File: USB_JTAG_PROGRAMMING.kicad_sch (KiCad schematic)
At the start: 85 parts, among them J16 10118194-0001LF, U3 FT2232HQ, U36 MIC5504-3.3YM5-TR, U37 93LC56BT-I/OT, U38 KC2016K12.0000C1GE00, U39 SN74LVC1T45DBVR, U40 NC7WZ07P6X, U41 NC7SZ125M5X, U42 SN74LVC1T45DBVR, U43 SN74LVC1T45DBVR, U44 SN74LVC1T45DBVR, U45 SN74LVC1T45DBVR, U46 NC7WZ126K8X, U47 NC7WZ126K8X

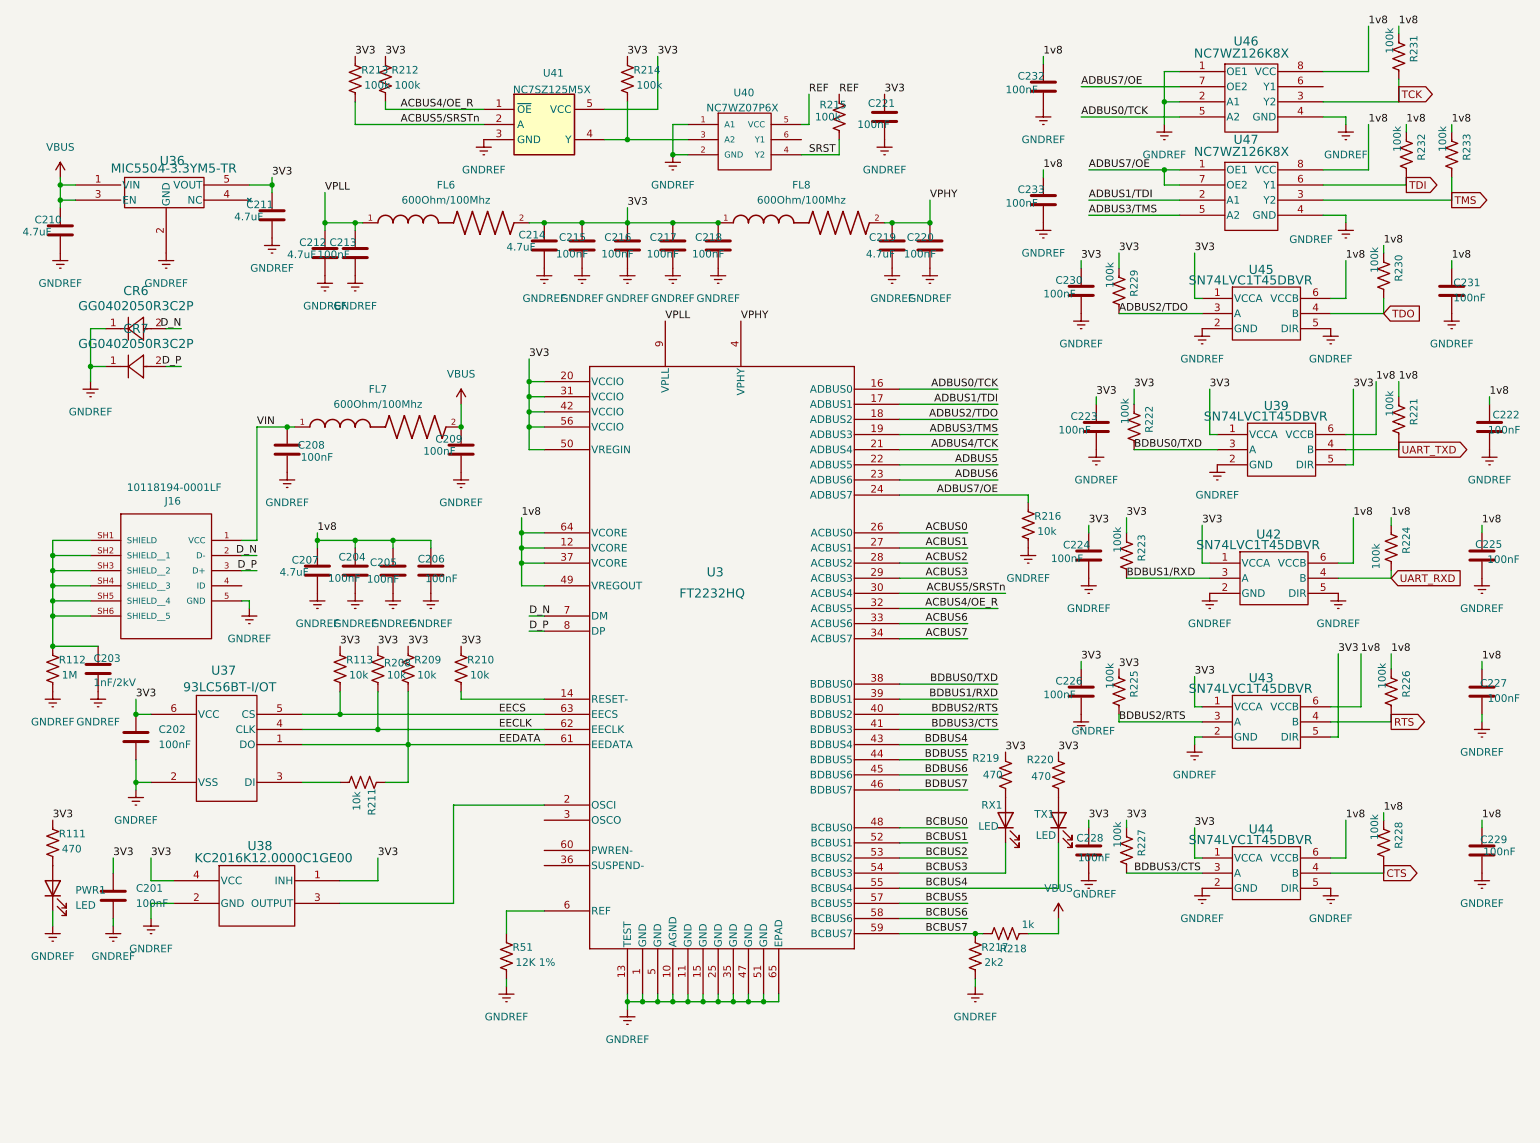
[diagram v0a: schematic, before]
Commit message: ready for manufacturing
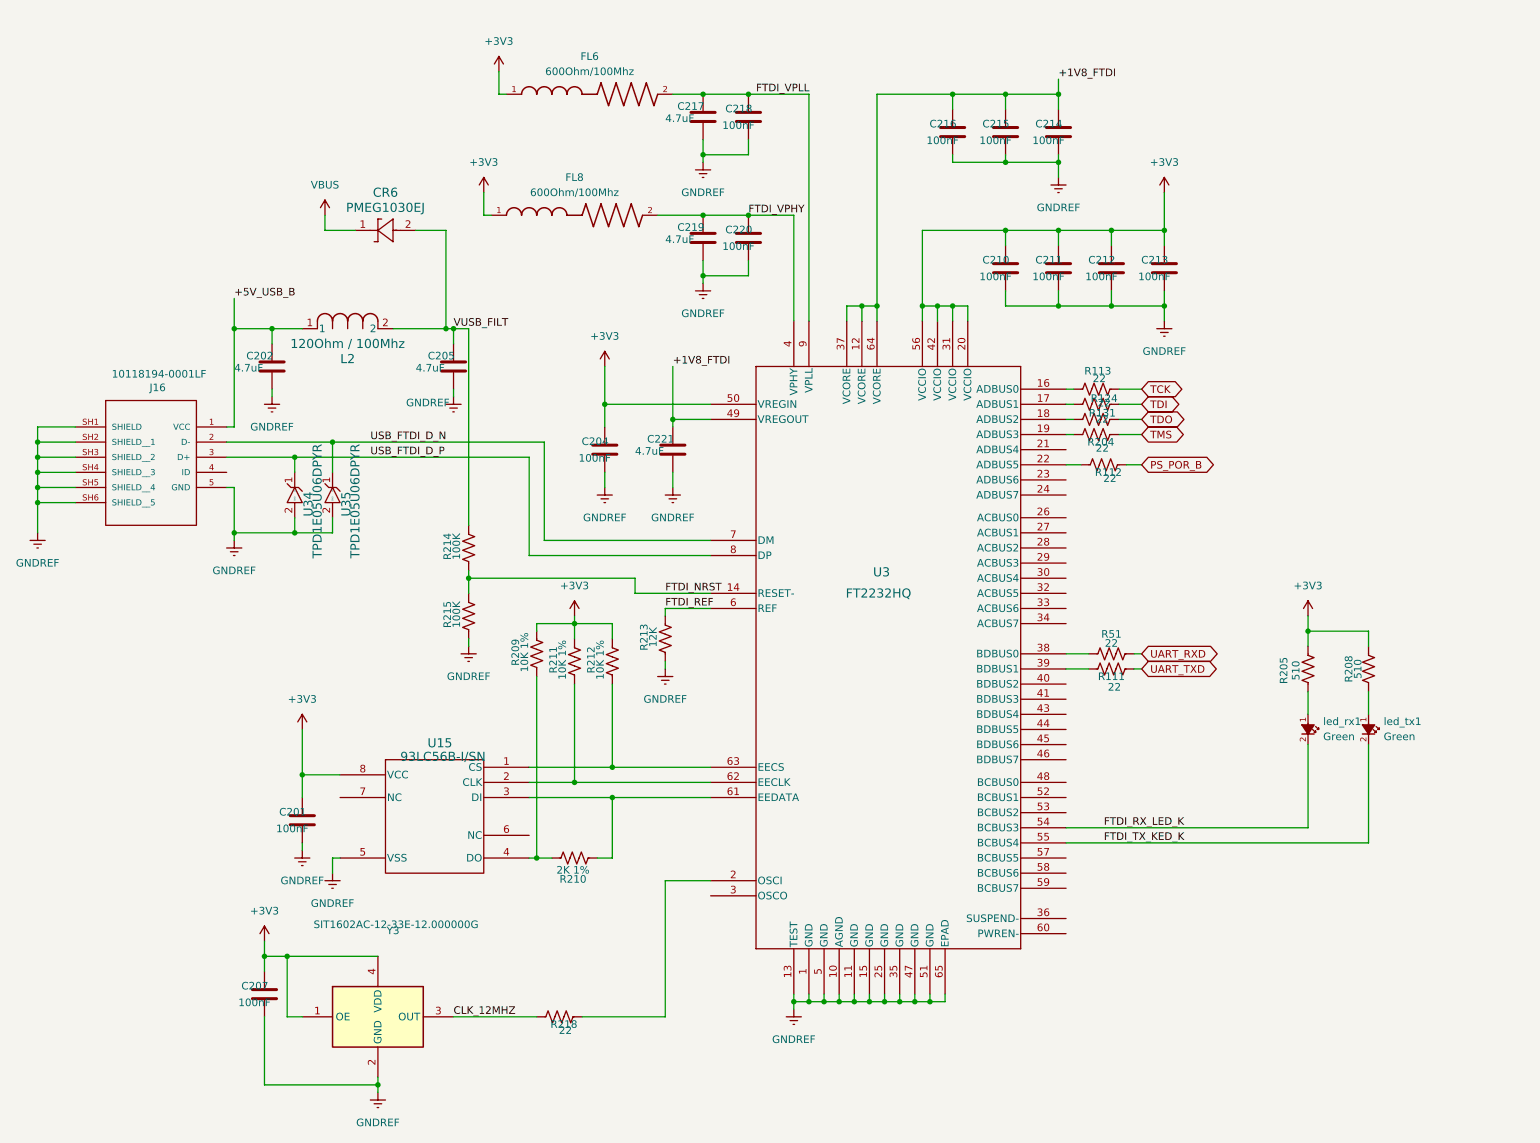
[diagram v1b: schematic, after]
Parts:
- removed C203: 1nF/2kV, footprints:C_1210_3225Metric, symbol Device:C
- removed C206, C208, C209, C222, C223, C224, C225, C226, C227, C228, C229, C230, C231, C232, C233: 100nF, footprints:C_0201_0603Metric, symbol Device:C
- removed CR6, CR7: GG0402050R3C2P, footprints:CR_050R3C2P_AVX, symbol GG0402050R3C2P:GG0402050R3C2P
- removed FL7: 600Ohm/100Mhz, footprints:BEADC1608X95N, symbol BLM18AG601SZ1D:BLM18AG601SZ1D
- removed PWR1, RX1, TX1: LED, footprints:LED_0402_1005Metric, symbol Device:LED
- removed R216: 10k, footprints:R_0402, symbol Device:R_US
- removed R217: 2k2, footprints:R_0402, symbol Device:R_US
- removed R219, R220: 470, footprints:R_0402, symbol Device:R_US
- removed R221, R222, R223, R224, R225, R226, R227, R228, R229, R230, R231, R232, R233: 100k, footprints:R_0402, symbol Device:R_US
- removed U36: MIC5504-3.3YM5-TR, footprints:SOT-23-5_MC_MCH, symbol MIC5504_3_3YM5_TR:MIC5504-3.3YM5-TR
- removed U37: 93LC56BT-I/OT, footprints:SOT-23-6_MC_MCH, symbol 93LC56BT_I_OT:93LC56BT-I_OT
- removed U38: KC2016K12.0000C1GE00, footprints:KC2016K_KYO, symbol KC2016K12-0000C1GE00:KC2016K12.0000C1GE00
- removed U39, U42, U43, U44, U45: SN74LVC1T45DBVR, footprints:DBV0006A_L, symbol SN74LVC1T45DBVR:SN74LVC1T45DBVR
- removed U40: NC7WZ07P6X, footprints:NC7WZ07P6X, symbol NC7WZ07P6X:NC7WZ07P6X
- removed U41: NC7SZ125M5X, footprints:SC-74A_318BQ_ONS, symbol 74xGxx:NC7SZ125M5X
- removed U46, U47: NC7WZ126K8X, footprints:US8-8_2P1X2P4_ONS, symbol NC7WZ126:NC7WZ126K8X
- added CR6: PMEG1030EJ, footprints:SOD323F_NXP, symbol PMEG1030EJ:PMEG1030EJ
- added L2: 120Ohm / 100Mhz, footprints:IND_BLM18_0603_MUR, symbol BLM18AG121SN1D:BLM18AG121SN1D
- added R124, R131, R204: 22, footprints:R_0201_0603Metric, symbol Device:R_US
- added R205: 510, footprints:R_0201_0603Metric, symbol Device:R_US
- added U15: 93LC56B-I/SN, footprints:SOIC8-N_MC_MCH, symbol 93LC56B-I-SN:93LC56B-I_SN
- added U34, U35: TPD1E05U06DPYR, footprints:DIO_TPD1E05U06DPYR, symbol TPD1E05U06DPYR:TPD1E05U06DPYR
- added Y3: SIT1602AC-12-33E-12.000000G, footprints:SIT1602AC1233E12000000G, symbol SIT1602AC-12-33E-12_000000G:SIT1602AC-12-33E-12.000000G
- added led_rx1, led_tx1: Green, footprints:LED_0402_1005Metric, symbol Aquiot:LED
- C201, C204, C213, C215, C216, C218, C220: LCSC PN c1525 -> c307380
- C202, C205, C217, C221: value 100nF -> 4.7uF; footprint footprints:C_0201_0603Metric -> footprints:C_0402; LCSC PN c1525 -> C2858031
- C207, C210, C211, C212, C214: value 4.7uF -> 100nF; footprint footprints:C_0402 -> footprints:C_0201_0603Metric; LCSC PN c23733 -> c307380
- C219: LCSC PN c23733 -> C2858031
- J16: LCSC PN C132563 -> (none)
- R111: value 470 -> 22; footprint footprints:R_0402 -> footprints:R_0201_0603Metric; LCSC PN C114877 -> C270355
- R112: value 1M -> 22; footprint footprints:R_0402 -> footprints:R_0201_0603Metric; LCSC PN C138033 -> C270355
- R113: value 10k -> 22; footprint footprints:R_0402 -> footprints:R_0201_0603Metric; LCSC PN C60490 -> C270355
- R208: value 10k -> 510; footprint footprints:R_0402 -> footprints:R_0201_0603Metric; LCSC PN C60490 -> C713499
- R209, R211: value 10k -> 10K 1%
- R210: value 10k -> 2K 1%; LCSC PN C60490 -> C60488
- R212: value 100k -> 10K 1%; LCSC PN C60491 -> C60490
- R213: value 100k -> 12K; footprint footprints:R_0402 -> footprints:R_0201_0603Metric; LCSC PN C60491 -> C2092166
- R214, R215: value 100k -> 100K
- R218: value 1k -> 22; footprint footprints:R_0402 -> footprints:R_0201_0603Metric; LCSC PN c106235 -> C270355
- R51: value 12K 1% -> 22; footprint footprints:R_0402 -> footprints:R_0201_0603Metric; LCSC PN C114760 -> C270355
- U3: LCSC PN C193662 -> C3025148
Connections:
- net BDBUS0/TXD is gone; now on an unnamed net: U3.38 (BDBUS0)
- net REF is gone; now on net GNDREF: R215.1
- net GNDREF: now also J16.SH1 (SHIELD), J16.SH2 (SHIELD__1), J16.SH3 (SHIELD__2), J16.SH4 (SHIELD__3), J16.SH5 (SHIELD__4), J16.SH6 (SHIELD__5), R213.1, U15.5 (VSS), U34.2 (GND), U35.2 (GND), Y3.2 (GND); no longer R112.2, R51.2
- net TCK: now also R113.2
- net TDI: now also R124.2
- net TDO: now also R131.2
- net TMS: now also R204.2
- net UART_RXD: now also R51.2
- net UART_TXD: now also R111.2
- net VBUS: now also CR6.1; no longer C210.1, R218.2
- net at R51.1: no longer U3.6 (REF)
- net at U3.2 (OSCI): now also R218.2
- net +3V3: now reaches R211.2
- net +3V3: now also C201.1, C204.1, C207.1, C210.1, C211.1, C212.1, C213.1, FL6.1, FL8.1, R208.2, R209.2, R212.2, U3.20 (VCCIO), U3.31 (VCCIO), U3.42 (VCCIO), U3.50 (VREGIN), U3.56 (VCCIO), R205.2, U15.8 (VCC), Y3.1 (OE), Y3.4 (VDD)
- net at R210.2: now also R209.1, U15.4 (DO); no longer U3.14 (RESET-)
- net VUSB_FILT: now reaches R214.2
- net VUSB_FILT: now also C205.1, CR6.2, L2.2
- net 1v8 renamed +1V8_FTDI
- net +1V8_FTDI: now also C214.1, C215.1, C216.1, C221.1; no longer C204.1, C205.1, C207.1
- removed net 3V3: C201.1, C202.1, C211.1, C214.1, C215.1, C216.1, C217.1, C218.1, C221.1, FL6.2, FL8.1, R111.1, R113.1, R208.1, R209.1, R210.1, R212.1, R213.1, R214.1, U3.20 (VCCIO), U3.31 (VCCIO), U3.42 (VCCIO), U3.50 (VREGIN), U3.56 (VCCIO)
- net ACBUS0: no longer names the net of U3.26 (ACBUS0)
- net ACBUS1: no longer names the net of U3.27 (ACBUS1)
- net ACBUS2: no longer names the net of U3.28 (ACBUS2)
- net ACBUS3: no longer names the net of U3.29 (ACBUS3)
- net ACBUS4/OE_R: no longer names the net of U3.32 (ACBUS5)
- net ACBUS4/OE_R: no longer R212.2
- net ACBUS5/SRSTn: no longer names the net of U3.30 (ACBUS4)
- net ACBUS5/SRSTn: no longer R213.2
- net ACBUS6: no longer names the net of U3.33 (ACBUS6)
- net ACBUS7: no longer names the net of U3.34 (ACBUS7)
- net ADBUS0/TCK: no longer names the net of U3.16 (ADBUS0)
- net ADBUS0/TCK: now also R113.1
- net ADBUS1/TDI: no longer names the net of U3.17 (ADBUS1)
- net ADBUS1/TDI: now also R124.1
- net ADBUS2/TDO: no longer names the net of U3.18 (ADBUS2)
- net ADBUS2/TDO: now also R131.1
- net ADBUS3/TMS: no longer names the net of U3.19 (ADBUS3)
- net ADBUS3/TMS: now also R204.1
- net ADBUS4/TCK: no longer names the net of U3.21 (ADBUS4)
- net ADBUS5: no longer names the net of U3.22 (ADBUS5)
- net ADBUS5: now also R112.1
- net ADBUS6: no longer names the net of U3.23 (ADBUS6)
- net ADBUS7/OE: no longer names the net of U3.24 (ADBUS7)
- net BCBUS0: no longer names the net of U3.48 (BCBUS0)
- net BCBUS1: no longer names the net of U3.52 (BCBUS1)
- net BCBUS2: no longer names the net of U3.53 (BCBUS2)
- net BCBUS3 renamed FTDI_RX_LED_K
- net FTDI_RX_LED_K: now also led_rx1.2 (K)
- net BCBUS4 renamed FTDI_TX_KED_K
- net FTDI_TX_KED_K: now also led_tx1.2 (K)
- net BCBUS5: no longer names the net of U3.57 (BCBUS5)
- net BCBUS6: no longer names the net of U3.58 (BCBUS6)
- net BCBUS7: no longer names the net of U3.59 (BCBUS7)
- net BCBUS7: no longer R218.1
- net BDBUS1/RXD: no longer names the net of U3.39 (BDBUS1)
- net BDBUS1/RXD: now also R111.1
- net BDBUS2/RTS: no longer names the net of U3.40 (BDBUS2)
- net BDBUS3/CTS: no longer names the net of U3.41 (BDBUS3)
- net BDBUS4: no longer names the net of U3.43 (BDBUS4)
- net BDBUS5: no longer names the net of U3.44 (BDBUS5)
- net BDBUS6: no longer names the net of U3.45 (BDBUS6)
- net BDBUS7: no longer names the net of U3.46 (BDBUS7)
- net D_N renamed USB_FTDI_D_N
- net USB_FTDI_D_N: now also U35.1 (I/O)
- net D_P renamed USB_FTDI_D_P
- net USB_FTDI_D_P: now also U34.1 (I/O)
- net EECLK: no longer names the net of U3.62 (EECLK)
- net EECLK: now also R211.1, U15.2 (CLK); no longer R208.2
- net EECS: no longer names the net of U3.63 (EECS)
- net EECS: now also R212.1, U15.1 (CS); no longer R113.2
- removed net EEDATA: R209.2, R211.1, U3.61 (EEDATA)
- net SRST renamed FTDI_NRST
- net FTDI_NRST: now also R214.1, U3.14 (RESET-)
- net VIN renamed +5V_USB_B
- net +5V_USB_B: now also C202.1, L2.1
- net VPHY renamed FTDI_VPHY
- removed net VPLL: C212.1, C213.1, FL6.1, U3.9 (VPLL)
- new net: R210.1, U15.3 (DI), U3.61 (EEDATA)
- new net: R205.1, led_rx1.1 (A)
- new net: R208.1, led_tx1.1 (A)
- new net CLK_12MHZ: R218.1, Y3.3 (OUT)
- new net FTDI_REF: R213.2, U3.6 (REF)
- new net FTDI_VPLL: C217.1, C218.1, FL6.2, U3.9 (VPLL)
- new net PS_POR_B: R112.2
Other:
- moved on the sheet: J16, U3
